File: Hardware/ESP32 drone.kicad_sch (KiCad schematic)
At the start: 74 parts, among them IC1 TP4056, J1 USB_C_Receptacle_USB2.0, J2 Conn_01x02_Female, J3 B2B-PH-SM4-TB(LF)(SN), J4 Conn_01x02_Female, J5 Conn_01x02_Female, J6 Conn_01x02_Female, J8 Conn_01x06_Female, J9 Conn_01x06_Female, SW1 K3-1280S-F1, T1 SI2302DS-T1, T2 SI2302DS-T1, T3 SI2302DS-T1, T4 SI2302DS-T1, U1 100K, U2 AO3401, U3 MIC5219-3.3YM5, U4 100K, U5 100K, U6 CP2102N-Axx-xQFN28, U7 DDC114TU-7-F, U8 ESP32-WROOM-32, U9 MPU-6050

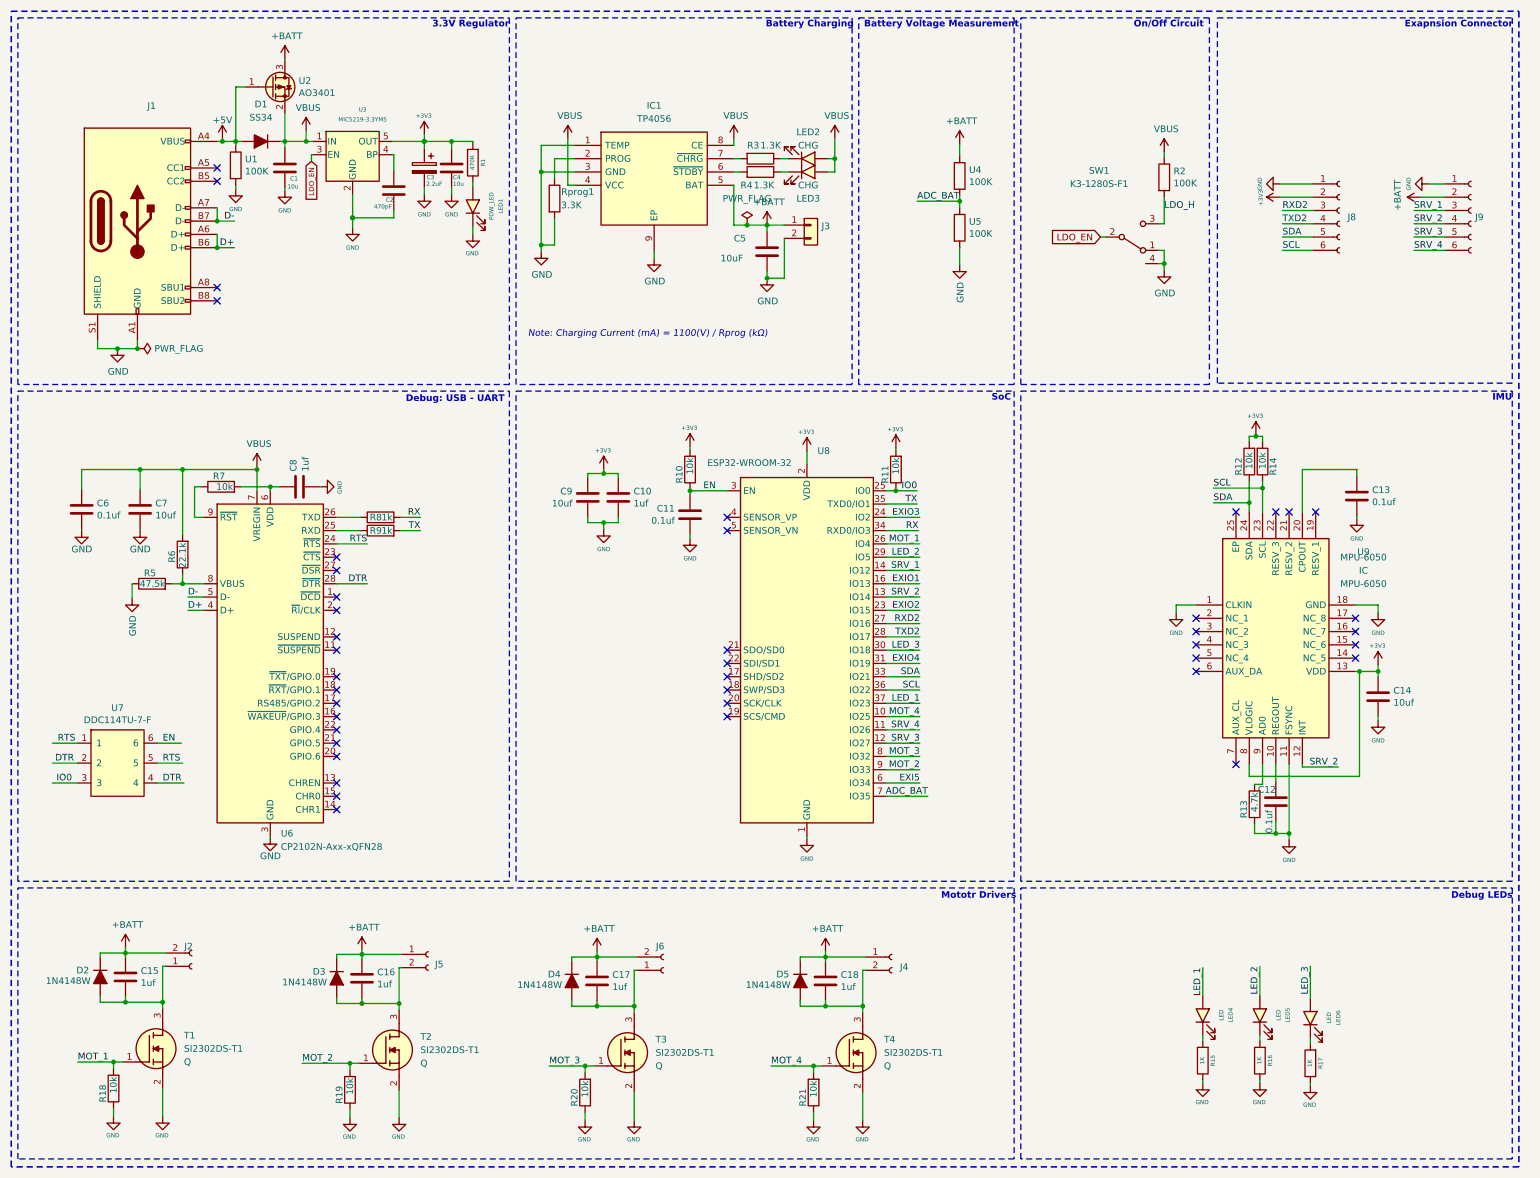
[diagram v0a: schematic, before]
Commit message: Organize drawings and BOM
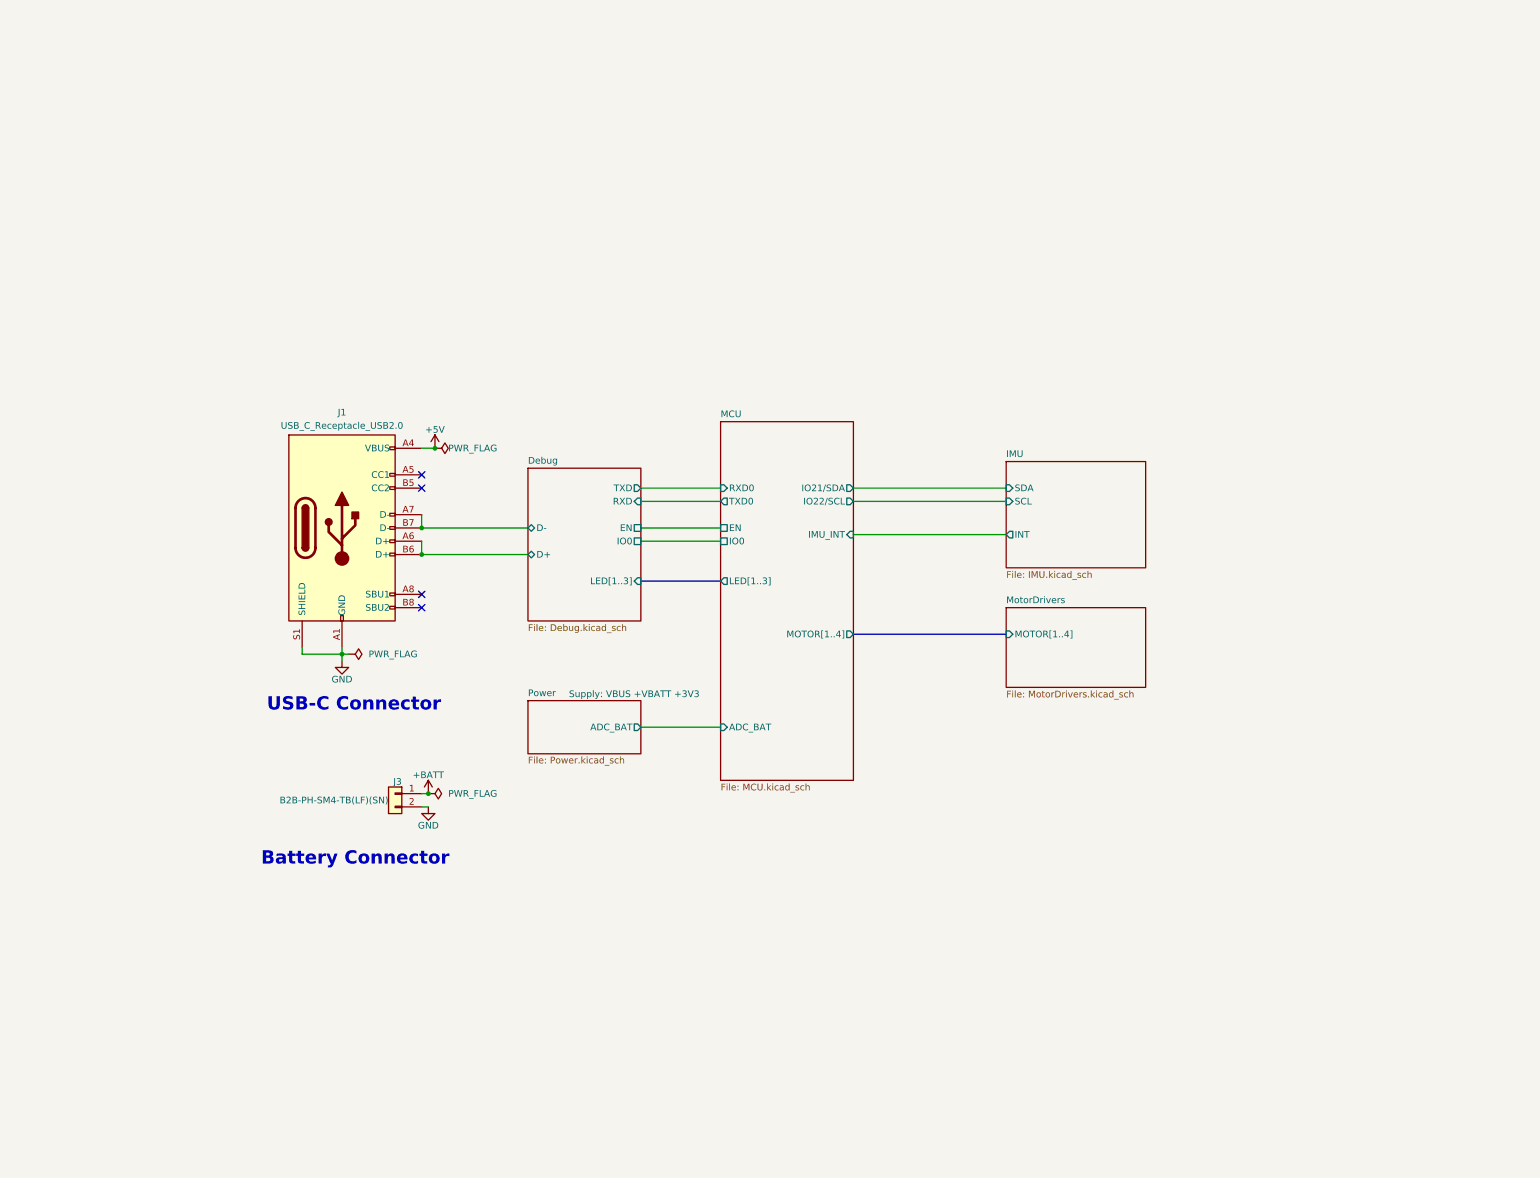
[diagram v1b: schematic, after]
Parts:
- removed C1, C4: 10u, Capacitor_SMD:C_0603_1608Metric, symbol Device:C
- removed C10, C15, C16, C17, C18, C8: 1uf, Capacitor_SMD:C_0603_1608Metric, symbol Device:C
- removed C11, C12, C13, C6: 0.1uf, Capacitor_SMD:C_0603_1608Metric, symbol Device:C
- removed C14, C7, C9: 10uf, Capacitor_SMD:C_0603_1608Metric, symbol Device:C
- removed C2: 470pF, Capacitor_SMD:C_0603_1608Metric, symbol Device:C
- removed C3: 2.2uF, Capacitor_SMD:C_0805_2012Metric, symbol Device:C_Polarized
- removed C5: 10uF, Capacitor_SMD:C_0603_1608Metric, symbol Device:C
- removed D1: SS34, Diode_SMD:D_SMA, symbol Diode:US1A
- removed D2, D3, D4, D5: 1N4148W, Diode_SMD:D_SOD-323, symbol Diode:1N4148W
- removed IC1: TP4056, tp4056:SOIC127P600X175-9N, symbol TP4056-42-ESOP8:TP4056-42-ESOP8
- removed J2, J4, J5, J6: Conn_01x02_Female, Connector_JST:JST_GH_SM02B-GHS-TB_1x02-1MP_P1.25mm_Horizontal, symbol Connector:Conn_01x02_Female
- removed J8, J9: Conn_01x06_Female, Connector_PinHeader_2.54mm:PinHeader_1x06_P2.54mm_Vertical, symbol Connector:Conn_01x06_Female
- removed LED1: POW_LED, LED_SMD:LED_0603_1608Metric, symbol Device:LED
- removed LED2, LED3: CHG, LED_SMD:LED_0603_1608Metric, symbol Device:LED
- removed LED4, LED5, LED6: LED, LED_SMD:LED_0603_1608Metric, symbol Device:LED
- removed R1: 470R, Resistor_SMD:R_0603_1608Metric, symbol Device:R
- removed R10, R11, R12, R14, R18, R19, R20, R21, R7: 10k, Resistor_SMD:R_0603_1608Metric, symbol Device:R
- removed R13: 4.7k, Resistor_SMD:R_0603_1608Metric, symbol Device:R
- removed R15, R16, R17: 1K, Resistor_SMD:R_0603_1608Metric, symbol Device:R
- removed R2, U1, U4, U5: 100K, Resistor_SMD:R_0603_1608Metric, symbol Device:R
- removed R3, R4: 1.3K, Resistor_SMD:R_0603_1608Metric, symbol Device:R
- removed R5: 47.5k, Resistor_SMD:R_0603_1608Metric, symbol Device:R
- removed R6: 22.1k, Resistor_SMD:R_0603_1608Metric, symbol Device:R
- removed R8, R9: 1k, Resistor_SMD:R_0603_1608Metric, symbol Device:R
- removed Rprog1: 3.3K, Resistor_SMD:R_0603_1608Metric, symbol Device:R
- removed SW1: K3-1280S-F1, ESP32_TouchDown_lib:slide switch spdt, symbol Switch:SW_SPDT
- removed T1, T2, T3, T4: SI2302DS-T1, SI2302DS-T1:SOT95P237X112-3N, symbol SI2302DS-T1:SI2302DS-T1
- removed U2: AO3401, Package_TO_SOT_SMD:SOT-23, symbol ESP32_TouchDown:DMG3415U-7
- removed U3: MIC5219-3.3YM5, Package_TO_SOT_SMD:SOT-23-5, symbol Regulator_Linear:MIC5219-3.3YM5
- removed U6: CP2102N-Axx-xQFN28, Package_DFN_QFN:QFN-28-1EP_5x5mm_P0.5mm_EP3.35x3.35mm, symbol Interface_USB:CP2102N-Axx-xQFN28
- removed U7: DDC114TU-7-F, Package_TO_SOT_SMD:SOT-363_SC-70-6, symbol downloader-rescue:DDC114TU-7-F-my
- removed U8: ESP32-WROOM-32, RF_Module:ESP32-WROOM-32, symbol RF_Module:ESP32-WROOM-32
- removed U9: MPU-6050, MPU6050:MPU6050, symbol MPU-6050:MPU-6050
- J1: symbol downloader-rescue:USB_C_Receptacle_USB2.0-Connector -> Connector:USB_C_Receptacle_USB2.0_16P; Manufacturer_Name (none) -> XUNPU
- J3: Manufacturer_Name (none) -> JST
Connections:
- net D+ renamed Debug/D+
- net D- renamed Debug/D-
- no-connect marks 42 -> 4
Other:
- added sheet Debug (Debug.kicad_sch)
- added sheet IMU (IMU.kicad_sch)
- added sheet MCU (MCU.kicad_sch)
- added sheet MotorDrivers (MotorDrivers.kicad_sch)
- added sheet Power (Power.kicad_sch)
- note added: "Battery Connector"
- note added: "USB-C Connector"
- note removed: "3.3V Regulator"
- note removed: "Battery Charging"
- note removed: "Battery Voltage Measurement"
- note removed: "Debug LEDs"
- note removed: "Debug: USB - UART"
- note removed: "Exapnsion Connector"
- note removed: "IMU"
- note removed: "Mototr Drivers"
- note removed: "Note: Charging Current (mA) = 1100(V) / Rprog (kΩ)"
- note removed: "On/Off Circuit"
- note removed: "SoC"
- company: Jobit Joseph -> (none)
- moved on the sheet: J1, J3
